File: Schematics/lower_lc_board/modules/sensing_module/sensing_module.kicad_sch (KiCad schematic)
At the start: 21 parts, among them J4 HALL-1, J5 HALL-2, Q3 2N7002, U11 SI2301CDS-T1-GE3, U9 ADC_ADS131M04IPWR

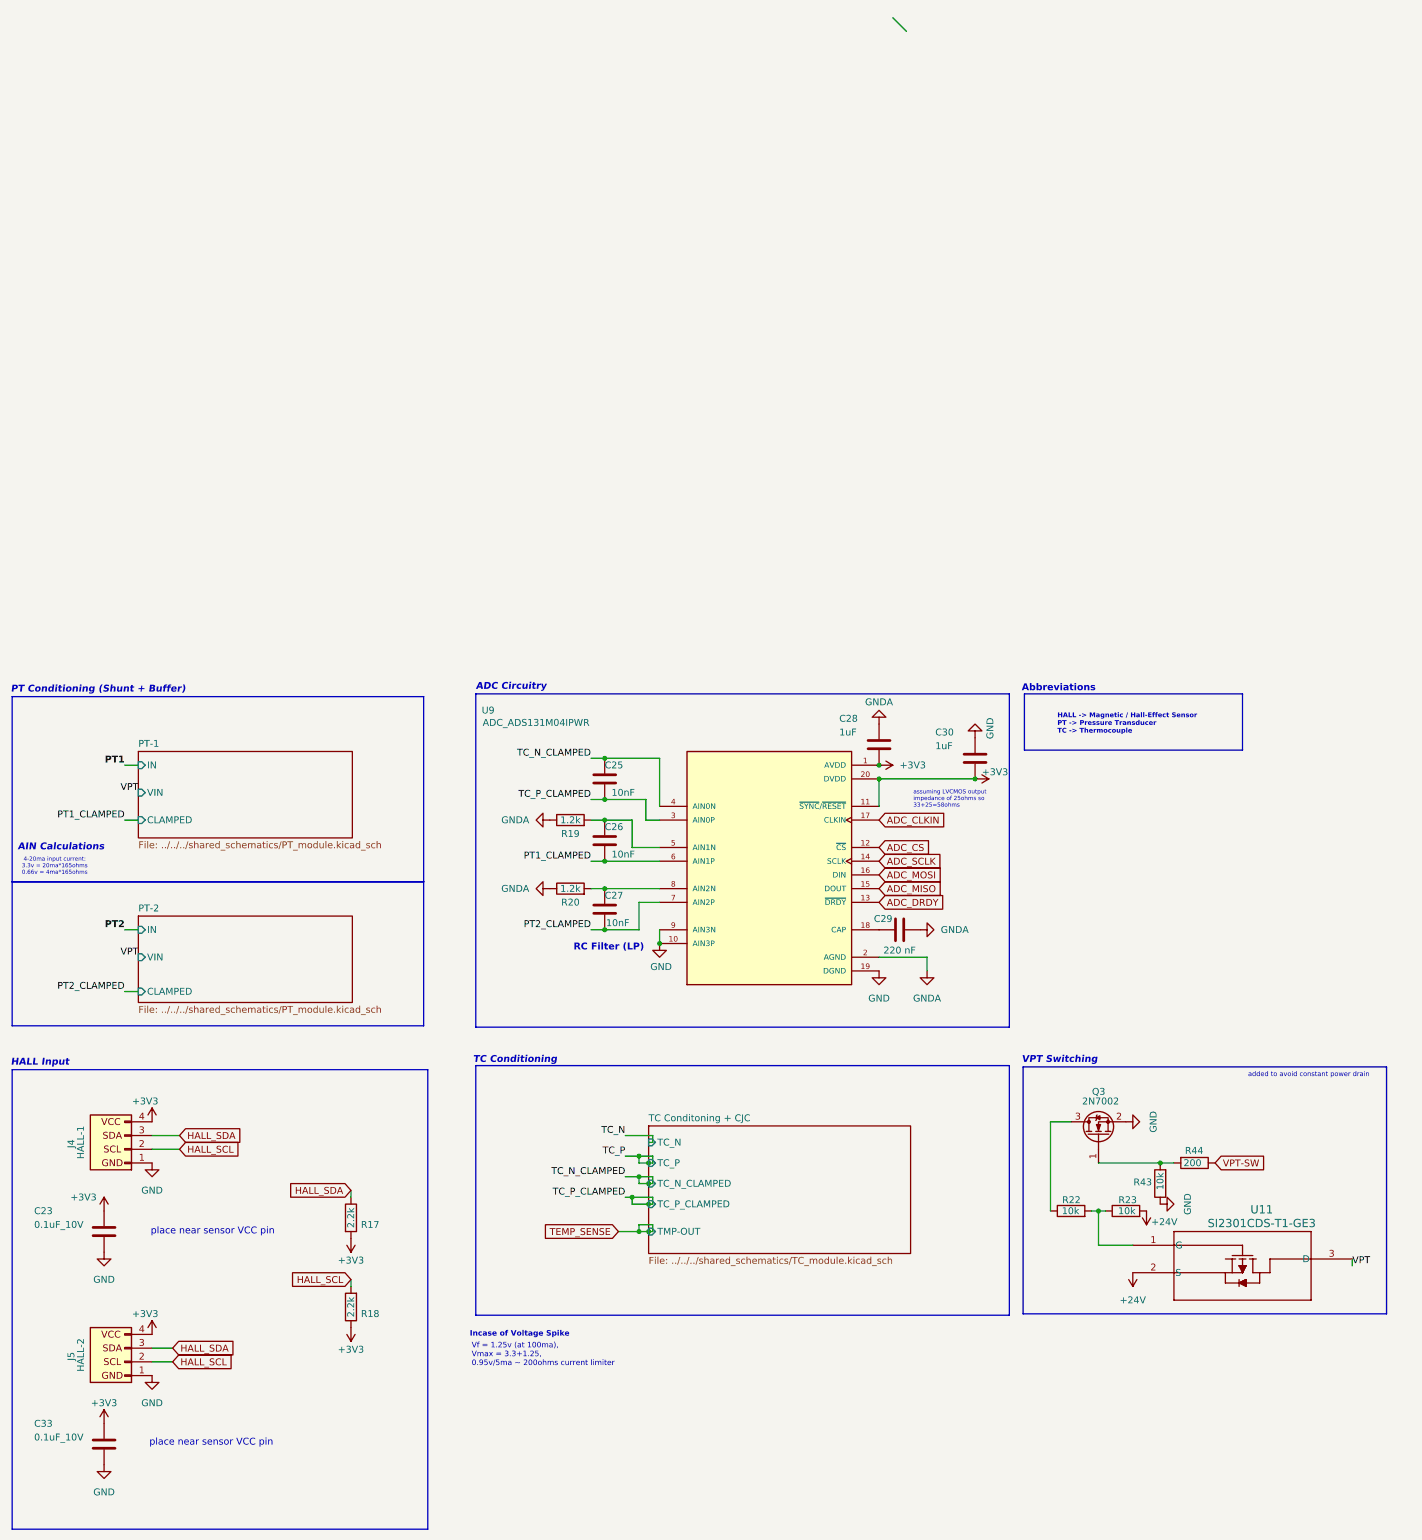
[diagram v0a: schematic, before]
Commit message: organizational work
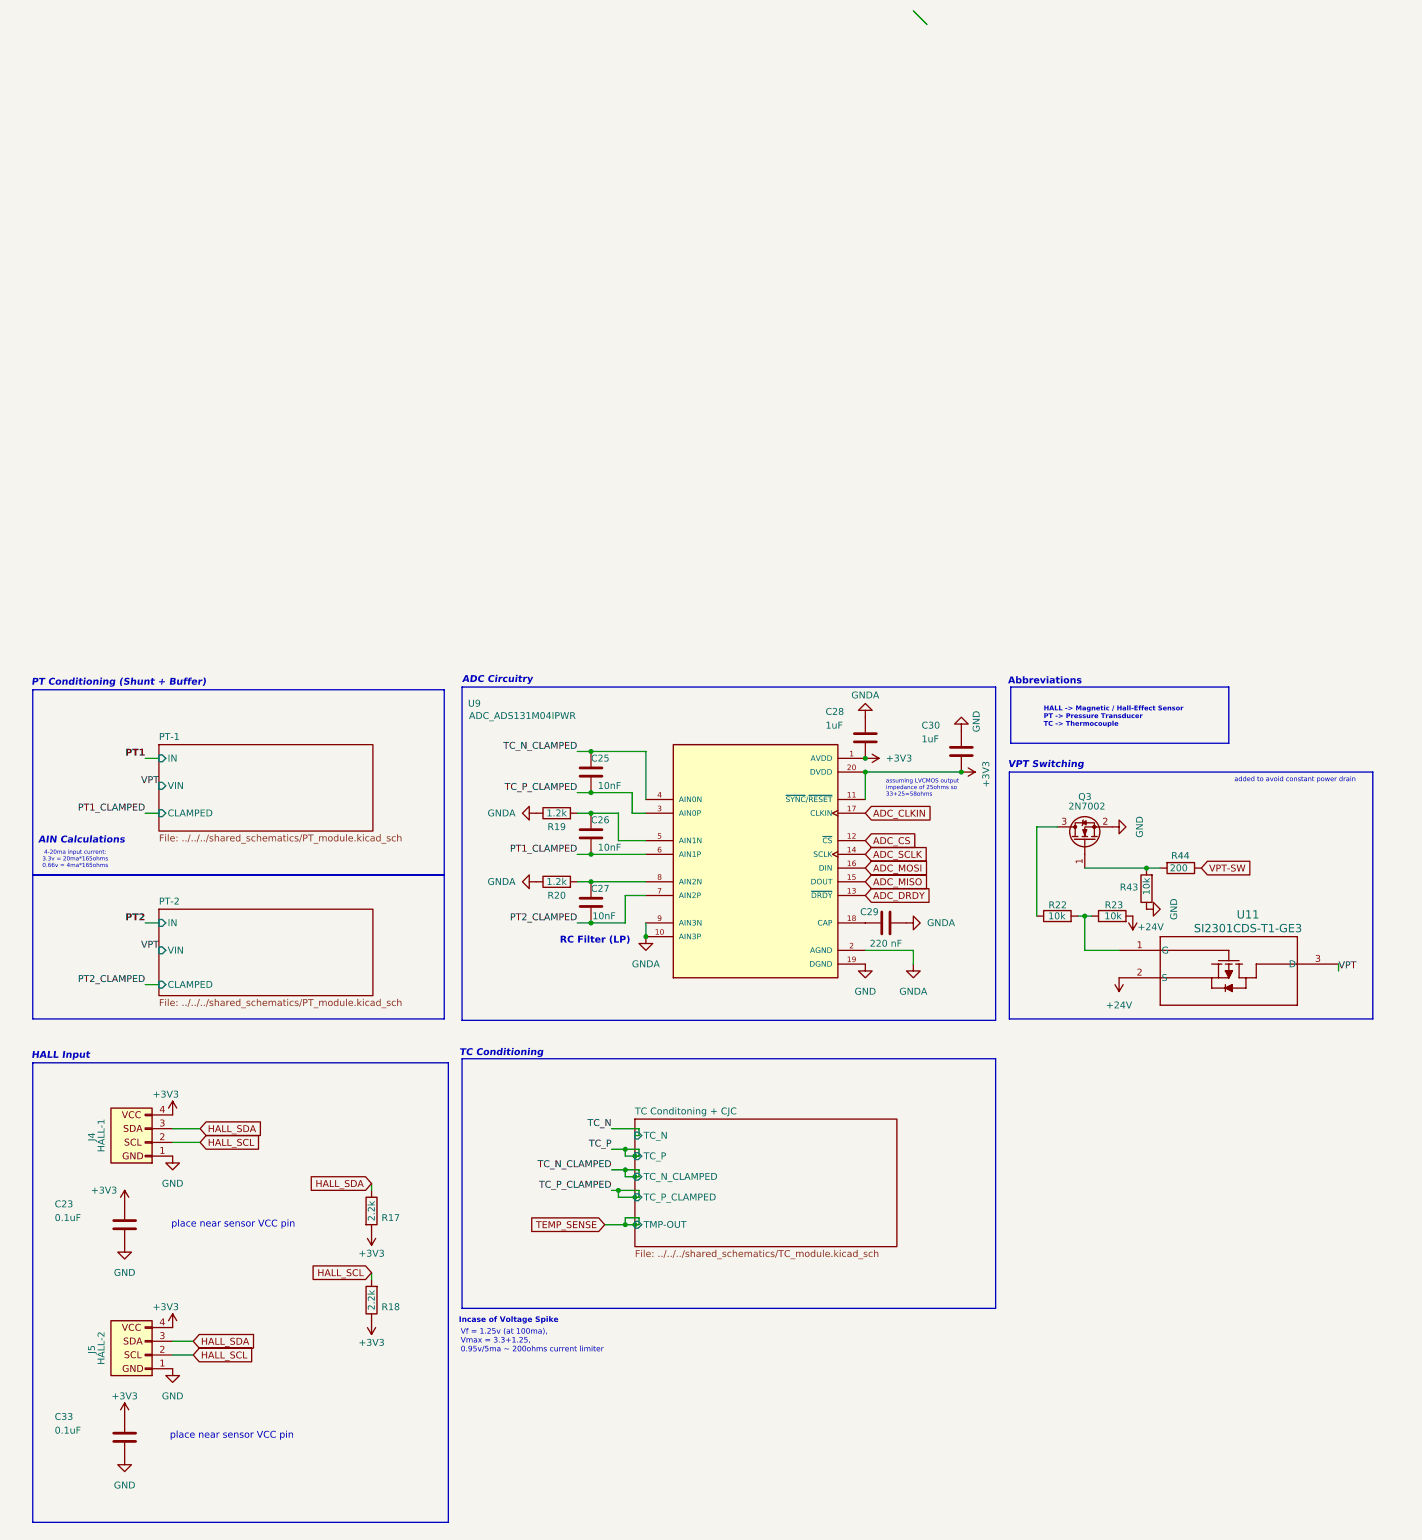
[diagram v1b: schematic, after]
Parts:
- C23, C33: value 0.1uF_10V -> 0.1uF
- C25, C26, C27: JLCPCB (none) -> C57112
- C28, C30: JLCPCB (none) -> C15849
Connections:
- net GND: no longer U9.10 (AIN3P), U9.9 (AIN3N)
- net GNDA: now also U9.10 (AIN3P), U9.9 (AIN3N)
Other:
- moved on the sheet: C23, C25, C26, C27, C28, C29, C30, C33, J4, J5, Q3, R17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
